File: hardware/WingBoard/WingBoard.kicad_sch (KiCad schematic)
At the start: 39 parts, among them J101 UPDI, J102 UART0, SW101 DIPA, SW102 DIPB, SW103 SW_SPST, U101 ATmega4809-A

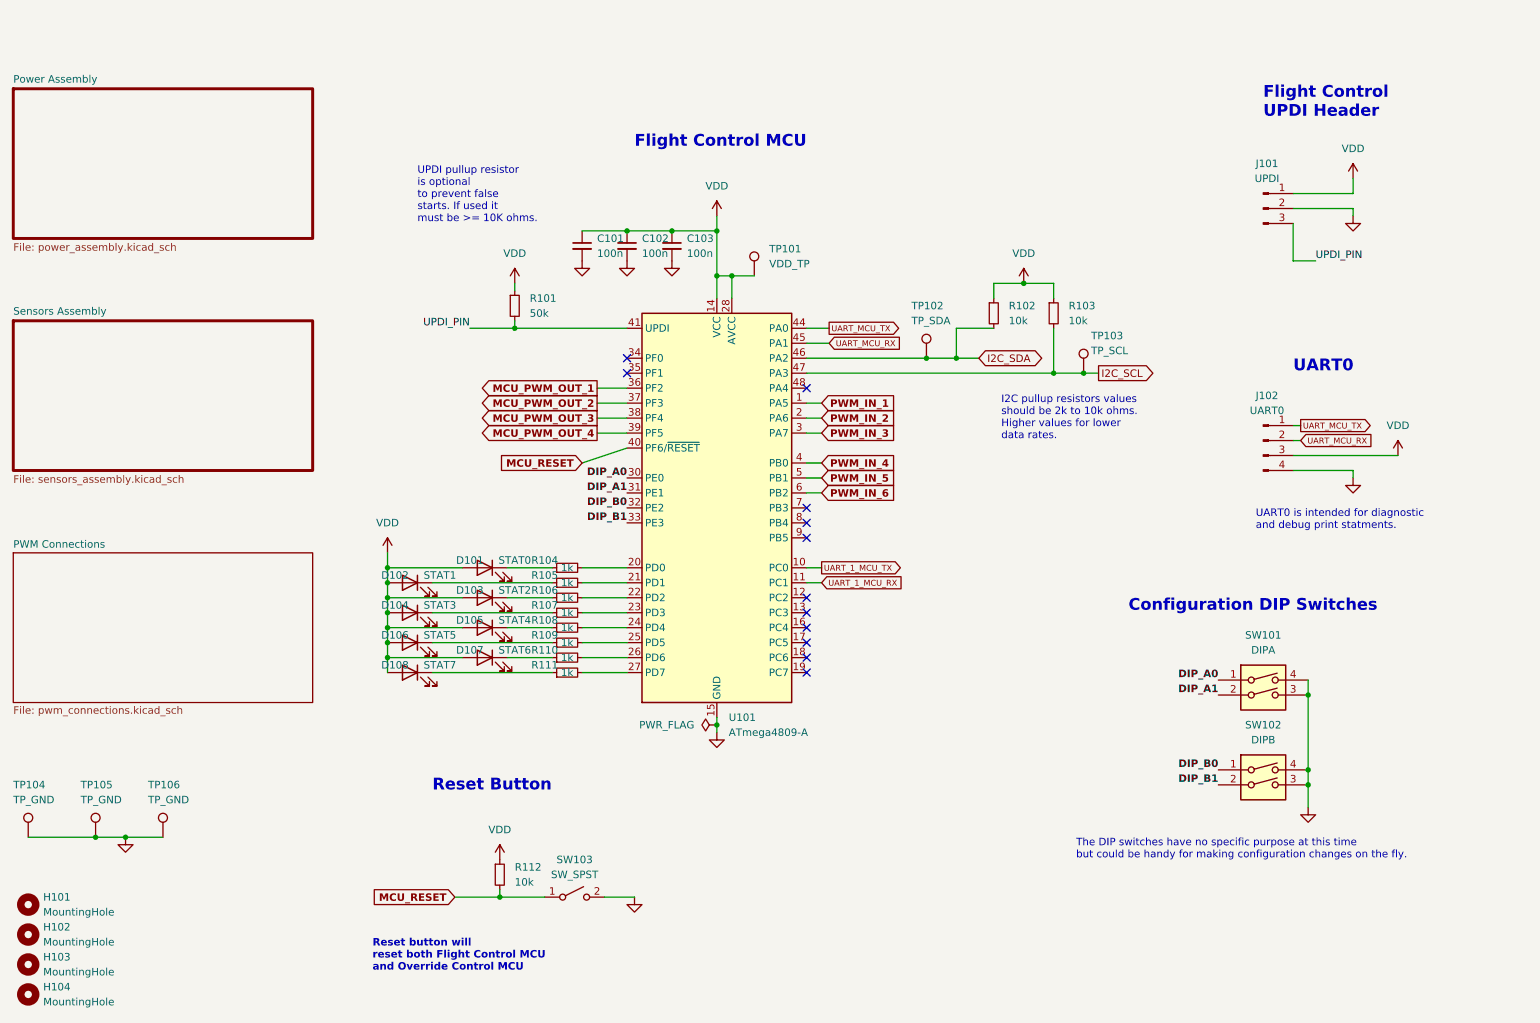
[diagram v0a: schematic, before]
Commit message: Hardware layout v0.1 complete.
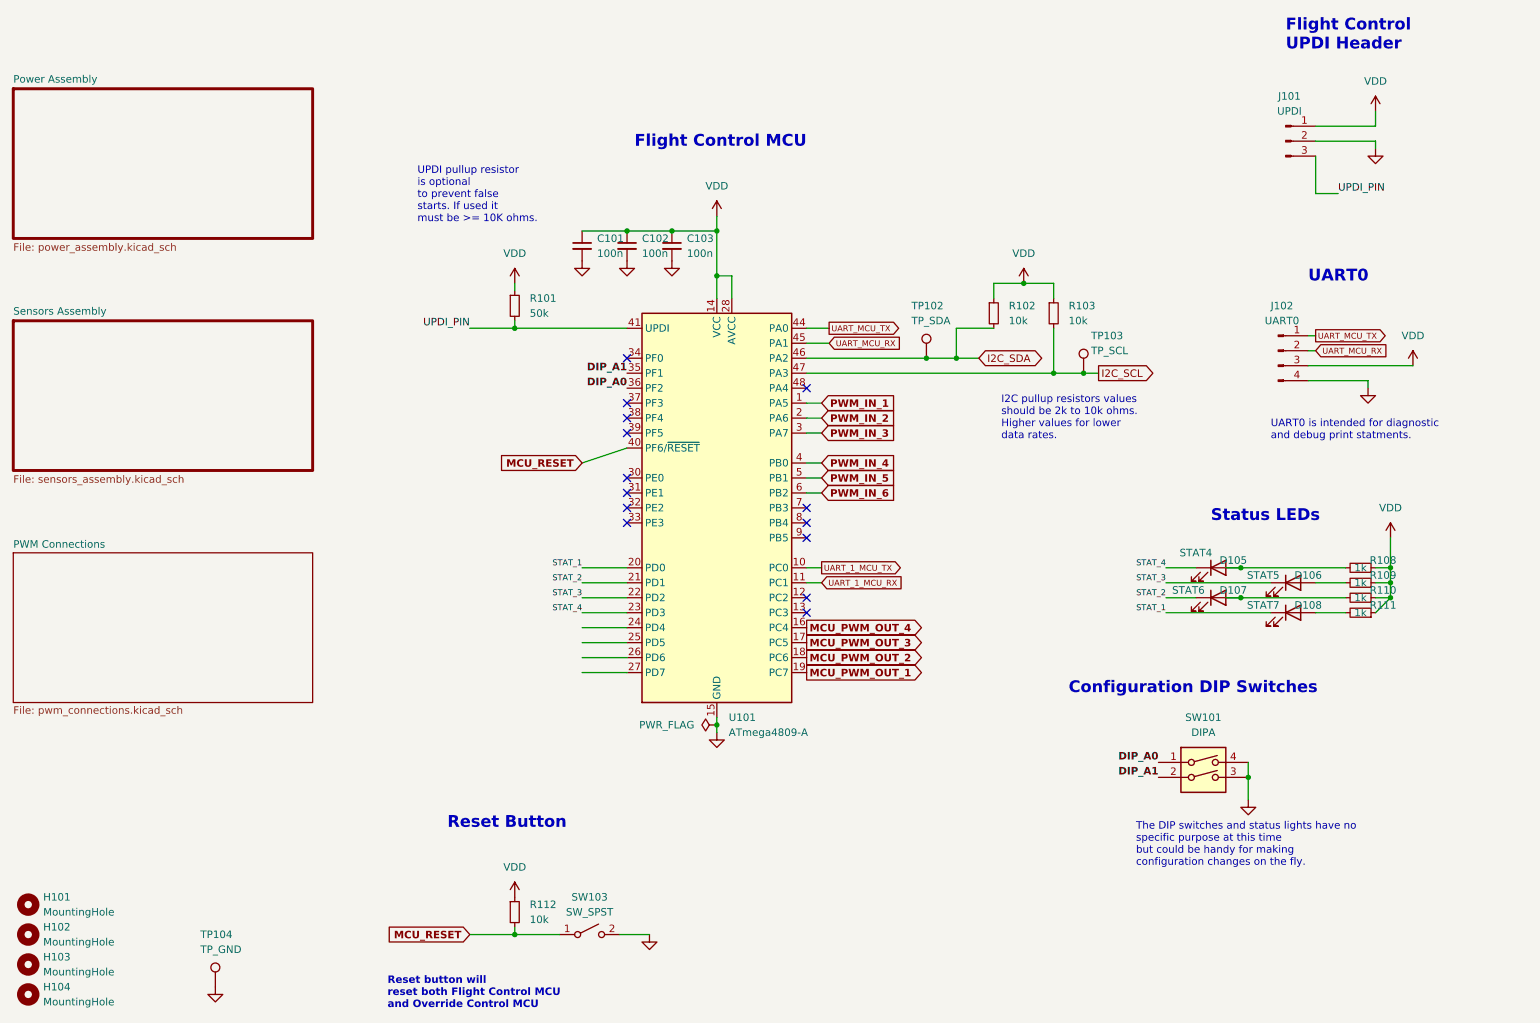
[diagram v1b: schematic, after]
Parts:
- removed D101: STAT0, LED_SMD:LED_0805_2012Metric_Pad1.15x1.40mm_HandSolder, symbol Device:LED
- removed D102: STAT1, LED_SMD:LED_0805_2012Metric_Pad1.15x1.40mm_HandSolder, symbol Device:LED
- removed D103: STAT2, LED_SMD:LED_0805_2012Metric_Pad1.15x1.40mm_HandSolder, symbol Device:LED
- removed D104: STAT3, LED_SMD:LED_0805_2012Metric_Pad1.15x1.40mm_HandSolder, symbol Device:LED
- removed R104, R105, R106, R107: 1k, Resistor_SMD:R_0805_2012Metric_Pad1.20x1.40mm_HandSolder, symbol Device:R_Small
- removed SW102: DIPB, Button_Switch_SMD:SW_DIP_SPSTx02_Slide_Copal_CHS-02B_W7.62mm_P1.27mm, symbol Switch:SW_DIP_x02
- removed TP101: VDD_TP, TestPoint:TestPoint_Pad_D1.5mm, symbol Connector:TestPoint
- removed TP105, TP106: TP_GND, TestPoint:TestPoint_Pad_D1.5mm, symbol Connector:TestPoint
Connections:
- net DIP_A0: now also U101.36 (PF2); no longer U101.30 (PE0)
- net DIP_A1: now also U101.35 (PF1); no longer U101.31 (PE1)
- net MCU_PWM_OUT_1: now also U101.19 (PC7); no longer U101.36 (PF2)
- net MCU_PWM_OUT_2: now also U101.18 (PC6); no longer U101.37 (PF3)
- net MCU_PWM_OUT_3: now also U101.17 (PC5); no longer U101.38 (PF4)
- net MCU_PWM_OUT_4: now also U101.16 (PC4); no longer U101.39 (PF5)
- net VDD: now also R108.1, R109.1, R110.1, R111.1; no longer D105.2 (A), D106.2 (A), D107.2 (A), D108.2 (A)
- net STAT_2: now reaches U101.21 (PD1)
- net STAT_2: now also D107.1 (K)
- net at R110.2: now also D107.2 (A); no longer U101.26 (PD6)
- net STAT_1: now reaches D108.1 (K)
- net STAT_1: now also U101.20 (PD0); no longer R111.1
- net at R111.2: now also D108.2 (A); no longer U101.27 (PD7)
- net STAT_3: now reaches D106.1 (K)
- net STAT_3: now also U101.22 (PD2); no longer R109.1
- net STAT_4: now reaches U101.23 (PD3)
- net STAT_4: now also D105.1 (K)
- net at R109.2: now also D106.2 (A); no longer U101.25 (PD5)
- net at R108.2: now also D105.2 (A); no longer U101.24 (PD4)
- net DIP_B0: no longer names the net of U101.32 (PE2)
- net DIP_B1: no longer names the net of U101.33 (PE3)
- no-connect marks 12 -> 14
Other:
- note added: "Status LEDs"
- note added: "The DIP switches and status lights have no specific purpose at this time but could be handy for making configuration changes on the fly."
- note removed: "The DIP switches have no specific purpose at this time but could be handy for making configuration changes on the fly."
- moved on the sheet: D105, D106, D107, D108, J101, J102, R108, R109, R110, R111, R112, SW101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
